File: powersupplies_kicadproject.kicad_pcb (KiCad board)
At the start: 6 copper layers, 160 x 99 mm, 18 parts, among them U2 TSR2-2465, U3 TSR2-2465

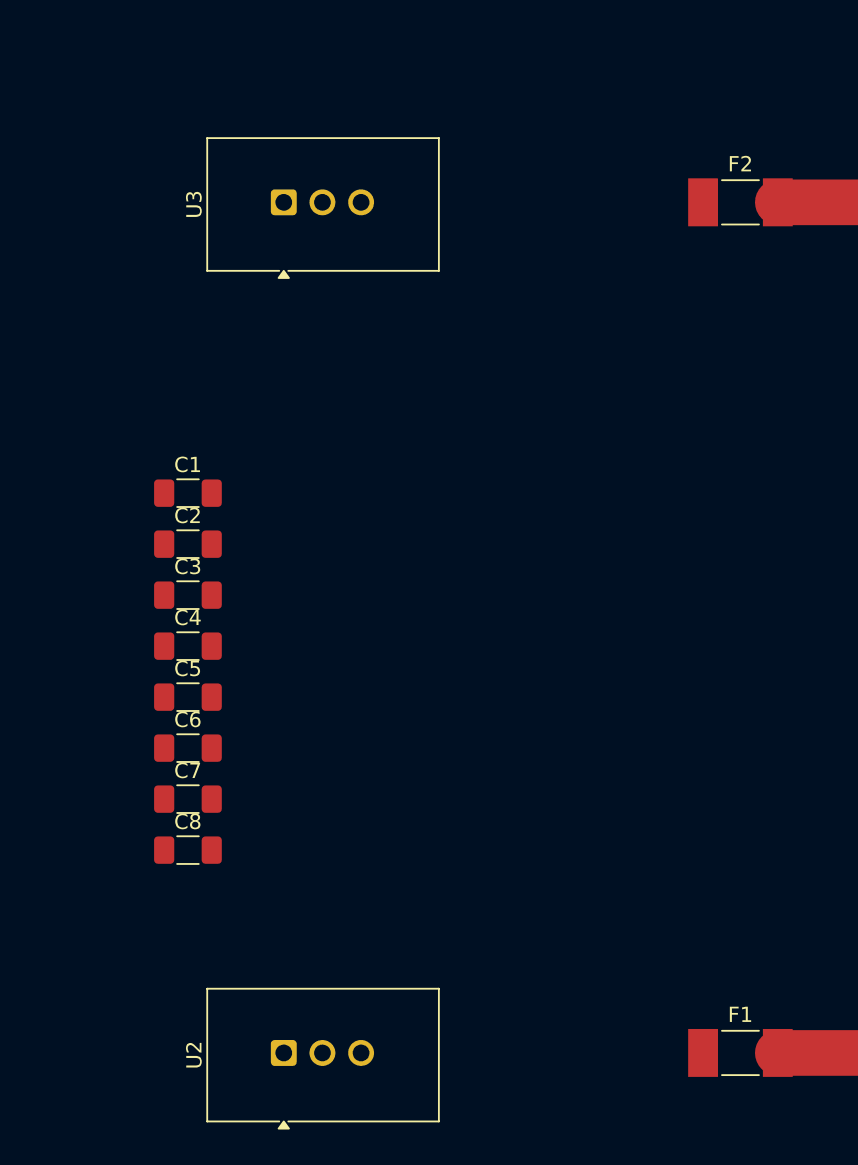
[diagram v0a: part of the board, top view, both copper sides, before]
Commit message: Save progress.
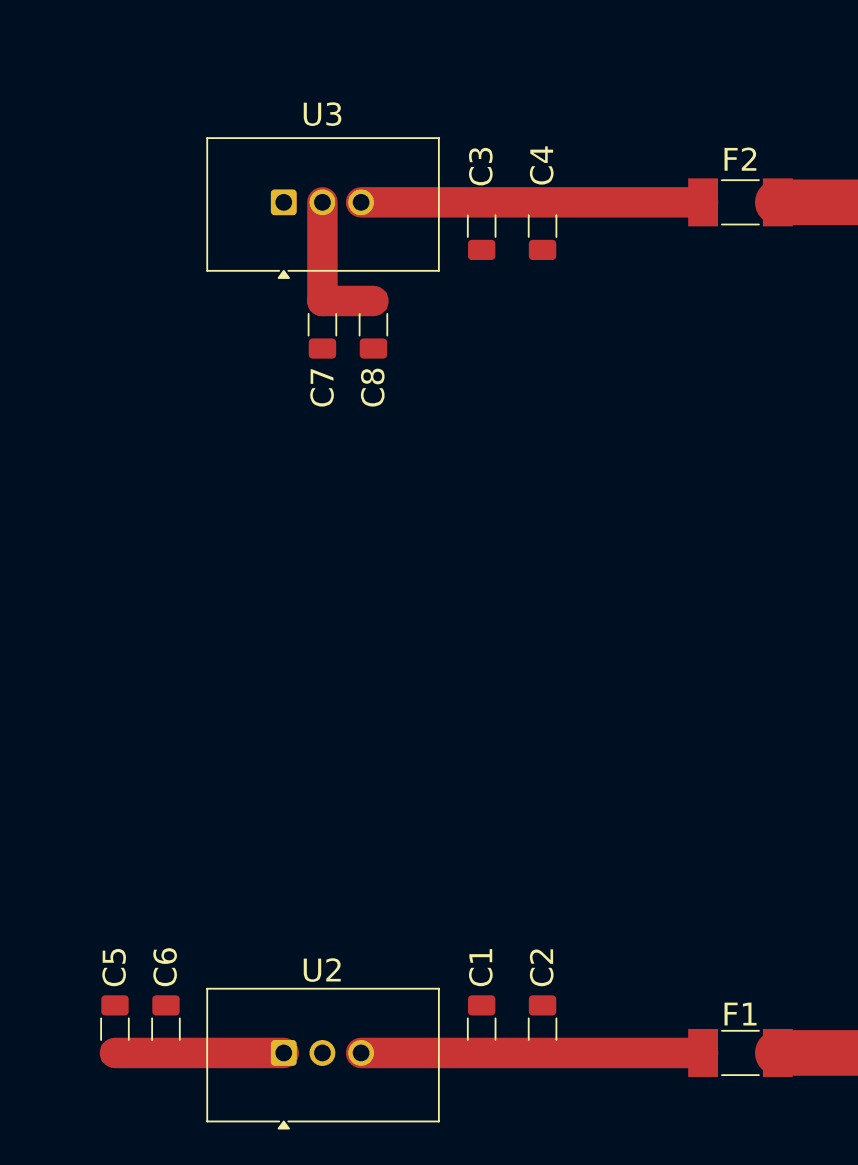
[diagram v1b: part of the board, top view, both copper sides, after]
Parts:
- moved C1 40.2 mm to (213.0, 127.6), turned to 90 degrees
- moved C2 39.5 mm to (217.0, 127.6), turned to 90 degrees
- moved C8 36.6 mm to (205.9, 81.4), turned to 90 degrees
- moved C4 36.1 mm to (217.0, 74.9), turned to 90 degrees
- moved C7 32.4 mm to (202.5, 81.4), turned to 90 degrees
- moved C3 31.0 mm to (213.0, 74.9), turned to 90 degrees
- moved C5 22.3 mm to (188.9, 127.6), turned to 90 degrees
- moved C6 18.5 mm to (192.3, 127.6), turned to 90 degrees
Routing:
- net Net-(U3-Vout): track 0.00 -> 22.5 mm
- net Net-(U2-Vout): track 0.00 -> 22.5 mm
- net /6.5V Dual Rail Power/+15V: track 5.08 -> 16.2 mm
- net /6.5V Dual Rail Power/-15V: track 5.08 -> 14.9 mm
